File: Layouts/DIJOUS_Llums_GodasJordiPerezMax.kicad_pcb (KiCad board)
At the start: 2 copper layers, 103.1 x 75.1 mm, 103 parts, among them J1 Conn_01x05_Socket, J2 Conn_01x03, J3 Conn_01x06, J4 Screw_Terminal_01x02, J5 Conn_01x05, J6 DE9_Plug, J7 Conn_01x02, J8 Conn_01x06_Socket, K1 G5LE-1 DC12, K2 G5LE-1 DC12, Q1 ZXTN19020DFFTA, Q2 ZXTN19020DFFTA, Q3 ZXTN19020DFFTA, Q4 Si7336ADP, Q5 Si7336ADP, Q6 ZXTN19020DFFTA, Q7 ZXTN19020DFFTA, Q8 Si7336ADP, Q9 Si7336ADP, U1 PCA9306D, U2 PIC18F2580-I/SO, U3 LM2596T-ADJ, U4 ADP7112ACBZ-3.3-R7, U5 MCP2551-I-SN, U6 ADM7172ACPZ-5.0-R7, U7 LT6202CS5

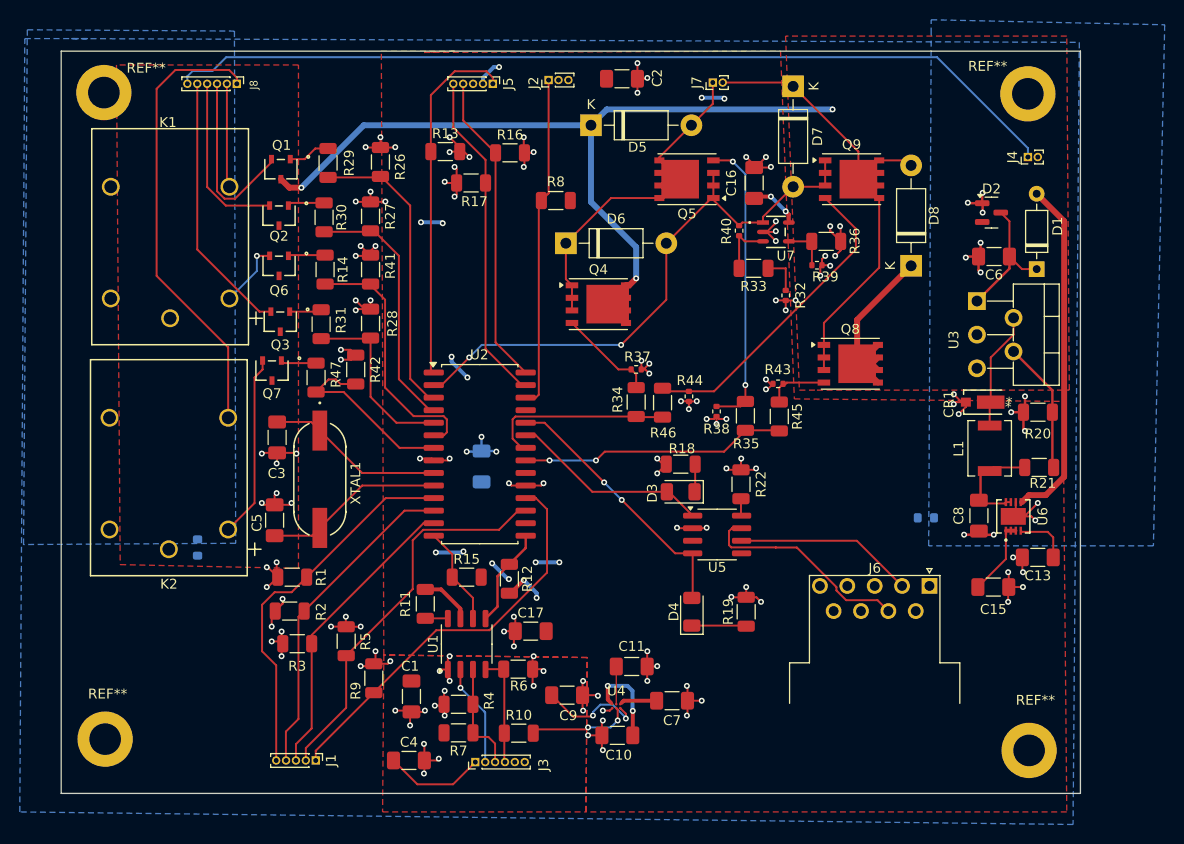
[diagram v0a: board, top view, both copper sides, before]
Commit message: Update Layout
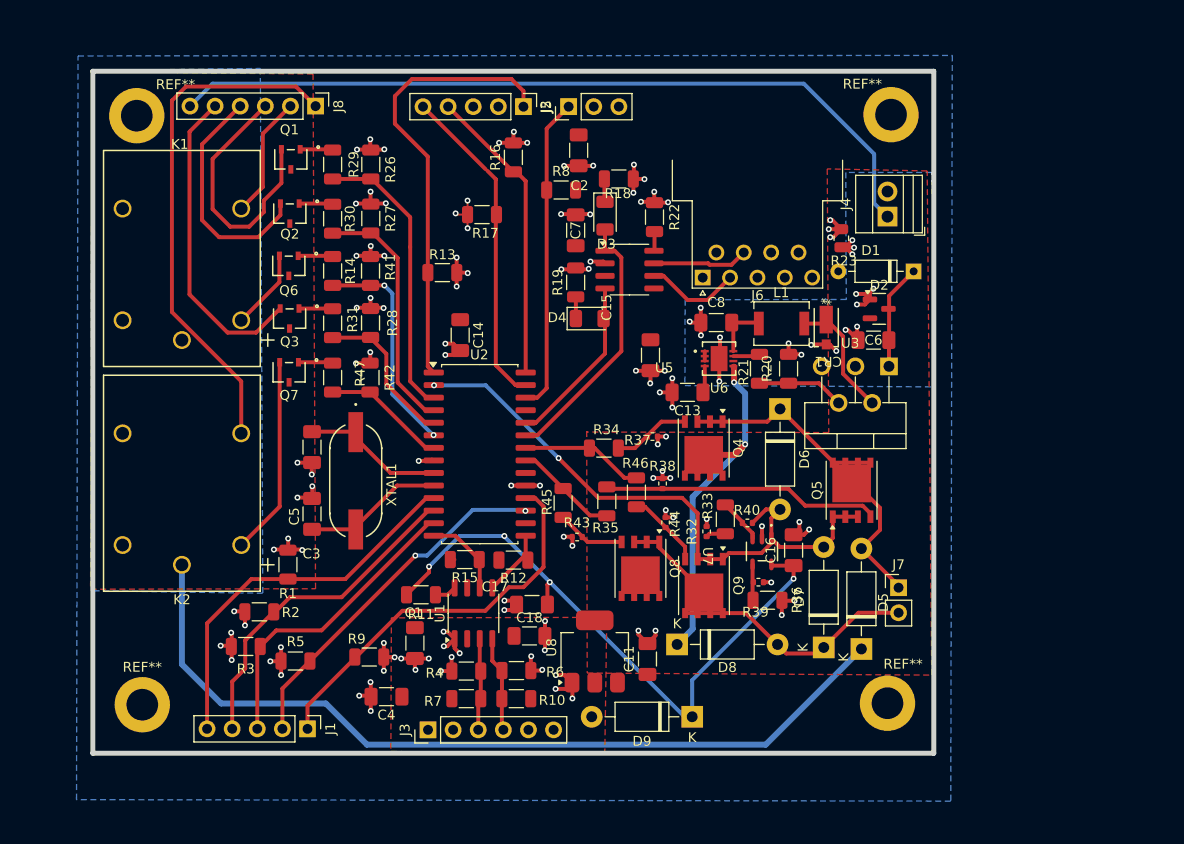
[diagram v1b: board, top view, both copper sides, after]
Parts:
- removed C10, C9: 2.2uF, Capacitor_SMD:C_1206_3216Metric_Pad1.33x1.80mm_HandSolder
- removed R48: 0, Resistor_SMD:R_0603_1608Metric
- removed the REF** at (150.5, 30.6)
- removed the REF** at (150.6, 97.0)
- removed the REF** at (57.1, 95.9)
- removed the REF** at (57.0, 30.5)
- removed U4: ADP7112ACBZ-3.3-R7, ADP7112ACBZ-3.3-R7:CB-6-15_ADI-M
- added C18: 100uF, Capacitor_SMD:C_1206_3216Metric_Pad1.33x1.80mm_HandSolder, F.Cu at (100.1, 85.4)
- added D9: 1N4002, Diode_THT:D_DO-41_SOD81_P10.16mm_Horizontal, F.Cu at (116.5, 93.6)
- added REF**: MountingHole_3.2mm_M3_DIN965_Pad, MountingHole:MountingHole_3.2mm_M3_DIN965_Pad, F.Cu at (60.4, 32.8)
- added REF**: MountingHole_3.2mm_M3_DIN965_Pad, MountingHole:MountingHole_3.2mm_M3_DIN965_Pad, F.Cu at (136.3, 92.3)
- added REF**: MountingHole_3.2mm_M3_DIN965_Pad, MountingHole:MountingHole_3.2mm_M3_DIN965_Pad, F.Cu at (60.9, 92.4)
- added REF**: MountingHole_3.2mm_M3_DIN965_Pad, MountingHole:MountingHole_3.2mm_M3_DIN965_Pad, F.Cu at (136.7, 32.7)
- added U8: TLV1117-33, Package_TO_SOT_SMD:SOT-223, F.Cu at (106.7, 87.0)
- C11: value 1nF -> 10uF
- C14: moved to F.Cu
- J1, J5: footprint Connector_PinHeader_1.00mm:PinHeader_1x05_P1.00mm_Vertical -> Connector_PinHeader_2.54mm:PinHeader_1x05_P2.54mm_Vertical
- J2: footprint Connector_PinHeader_1.00mm:PinHeader_1x03_P1.00mm_Vertical -> Connector_PinHeader_2.54mm:PinHeader_1x03_P2.54mm_Vertical
- J3, J8: footprint Connector_PinHeader_1.00mm:PinHeader_1x06_P1.00mm_Vertical -> Connector_PinHeader_2.54mm:PinHeader_1x06_P2.54mm_Vertical
- J4: footprint Connector_PinHeader_1.00mm:PinHeader_1x02_P1.00mm_Vertical -> TerminalBlock:TerminalBlock_Xinya_XY308-2.54-2P_1x02_P2.54mm_Horizontal
- J7: footprint Connector_PinHeader_1.00mm:PinHeader_1x02_P1.00mm_Vertical -> Connector_PinHeader_2.54mm:PinHeader_1x02_P2.54mm_Vertical
- R23: footprint Resistor_SMD:R_0603_1608Metric -> Resistor_SMD:R_0805_2012Metric; moved to F.Cu
- moved R23 72.2 mm to (131.6, 45.2), turned to -90 degrees
- moved D5 59.6 mm to (133.7, 86.8), turned to 90 degrees
- moved D7 56.9 mm to (129.8, 86.6), turned to 90 degrees
- moved J7 54.4 mm to (137.4, 80.6), turned to 0 degrees
- moved C7 48.6 mm to (104.7, 44.4), turned to 90 degrees
- moved D8 45.0 mm to (115.0, 86.3), turned to 0 degrees
- moved Q9 43.7 mm to (117.7, 80.3), turned to -90 degrees
- moved C15 41.9 mm to (112.3, 57.0), turned to -90 degrees
- moved C13 39.2 mm to (116.1, 60.8)
- moved J6 38.7 mm to (117.6, 49.2), turned to 180 degrees
- moved R19 37.5 mm to (104.7, 49.7)
- moved C16 37.4 mm to (126.8, 76.8)
- moved R36 36.8 mm to (124.2, 81.8)
- moved Q5 35.6 mm to (132.7, 70.7), turned to 90 degrees
- moved U6 33.8 mm to (119.3, 57.4), turned to 0 degrees
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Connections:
- net OSC1 renamed Net-(U2-OSC1/CLKI/RA7)
- net OSC2 renamed Net-(U2-OSC2/CLKO/RA6)
- C11 pad 1: Net-(U4-SS) -> +5V
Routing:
- net +3.3V: track 42.2 -> 0.20 mm, vias 5 -> 0
- net /BJTbase22: track 32.1 -> 7.85 mm
- net GND: track 168.1 -> 145.7 mm, vias 122 -> 106
- net +12V: track 141.0 -> 122.3 mm, vias 3 -> 2
- net Motor_in2: track 26.9 -> 10.5 mm, vias 2 -> 0
- net GNDPWR: track 118.5 -> 105.3 mm, vias 16 -> 17
- net CANH_O: track 21.9 -> 9.66 mm
- net CANRX: track 27.0 -> 17.5 mm, vias 2 -> 0
- net MCLR: track 36.4 -> 45.4 mm
- net Motor_o1: track 28.5 -> 37.5 mm
- net CANL_O: track 18.5 -> 9.65 mm
- net +5V: track 57.4 -> 66.0 mm, vias 22 -> 4
- net Motor_o2: track 42.6 -> 34.5 mm
- net Blinkers: track 18.5 -> 26.2 mm
- net Motor_in1: track 19.0 -> 12.5 mm
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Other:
- board size 103.1 x 75.1 mm -> 85.1 x 69 mm
